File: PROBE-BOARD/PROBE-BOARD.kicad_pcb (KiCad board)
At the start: 2 copper layers, 15 x 31.7 mm, 9 parts, among them J1 Conn_01x01, J2 Conn_01x01, SW1 SW_Push_Open

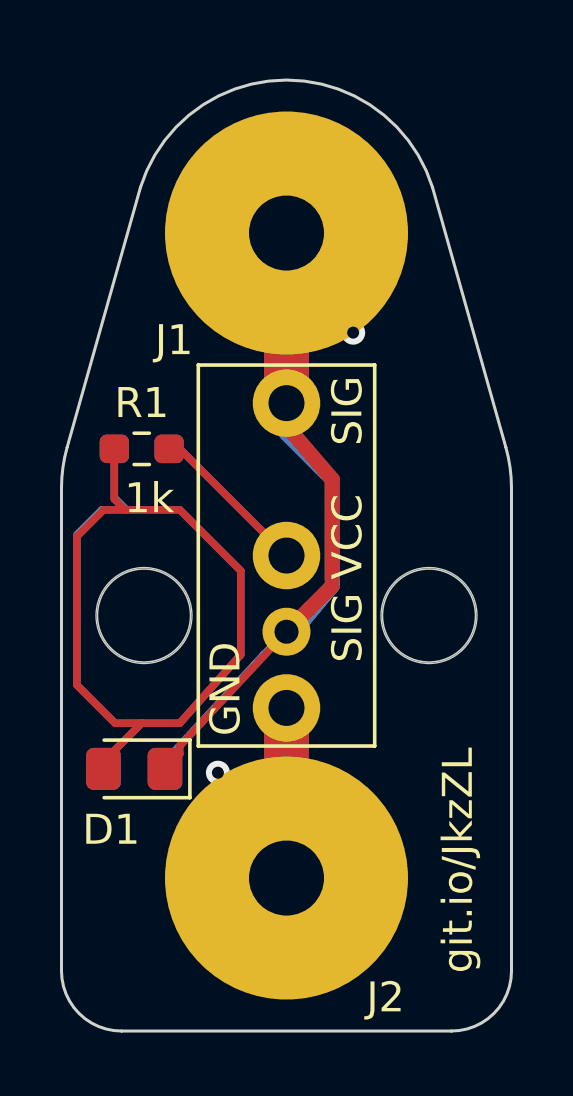
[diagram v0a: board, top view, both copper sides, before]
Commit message: move M3  mounting holes, recreted CAD, added gerbers
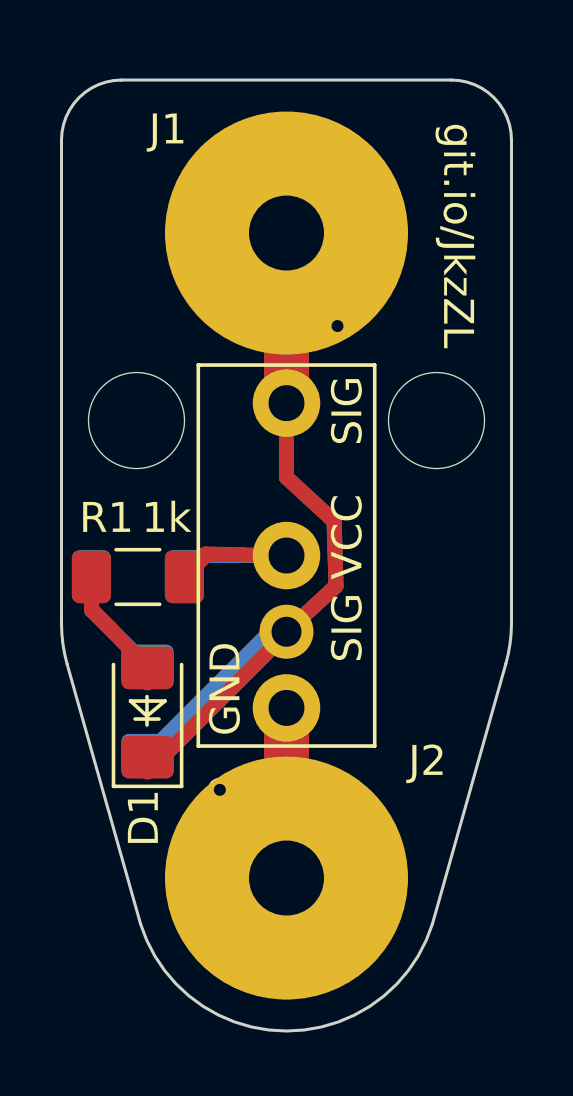
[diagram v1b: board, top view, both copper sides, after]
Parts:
- removed the REF** at (4.75, 2.00)
- removed the REF** at (-4.75, 2.00)
- added REF**: MountingHole_3.2mm_M3, MountingHole:MountingHole_3.2mm_M3, F.Cu at (5.00, -4.50)
- added REF**: MountingHole_3.2mm_M3, MountingHole:MountingHole_3.2mm_M3, F.Cu at (-5.00, -4.50)
- D1, D2: footprint LED_SMD:LED_0805_2012Metric_Pad1.15x1.40mm_HandSolder -> LED_SMD:LED_1206_3216Metric_Pad1.42x1.75mm_HandSolder
- R1, R2: footprint Resistor_SMD:R_0603_1608Metric_Pad0.98x0.95mm_HandSolder -> Resistor_SMD:R_1206_3216Metric_Pad1.30x1.75mm_HandSolder
- moved R1 4.27 mm to (-4.95, 0.71)
- moved R2 4.26 mm to (-4.95, 0.70)
- moved D2 1.99 mm to (-4.63, 5.17), turned to 90 degrees
- moved D1 1.93 mm to (-4.63, 5.23), turned to 90 degrees
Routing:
- net Net-(D2-Pad2): track 25.7 -> 3.76 mm
- net Net-(D1-Pad2): track 25.8 -> 4.28 mm
- net VCC: track 11.0 -> 7.79 mm
- net SIGNAL: track 44.5 -> 46.8 mm
- net GND: vias 0 -> 1
- net (no net): vias 1 -> 0
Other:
- outline, holes or cut-outs redrawn

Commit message: bOARD rev2
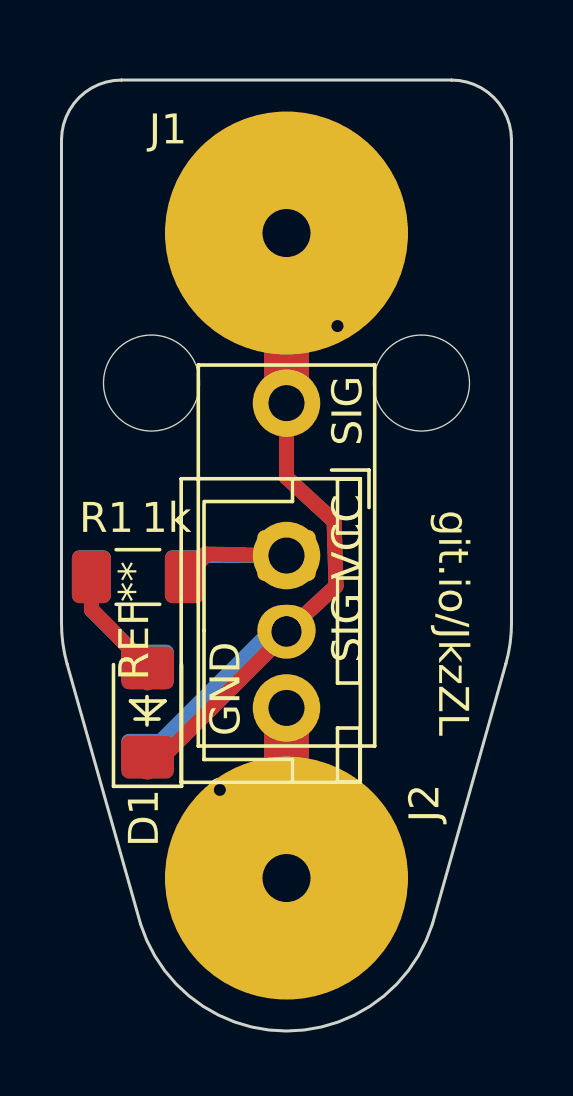
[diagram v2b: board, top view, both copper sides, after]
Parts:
- added REF**: JST-XH, mag-probe:JST-XH, F.Cu at (0.00, 0.00)
- added REF**: M3Heatsrt, mag-probe:M3Heatsrt, F.Cu at (-4.45, -5.80)
- added REF**: M3Heatsrt, mag-probe:M3Heatsrt, F.Cu at (4.45, -5.85)
- moved REF** 1.35 mm to (4.50, -5.75)
- moved REF** 1.31 mm to (-4.60, -5.75)
